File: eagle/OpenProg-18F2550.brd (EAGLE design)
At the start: 101.6 x 78.7 mm, 45 parts, among them J1 CONN-10P, J3 USB-SH, T1 BC557, T2 BC557, T3 BC547, T4 BC547, U1 PIC18F2550-I/SP-V, X1 12MHz

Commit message: ...
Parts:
- L1: value (none) -> 100µH
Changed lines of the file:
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@@
 <element name="J1" library="pinconn" package="CONN-10P" value="CONN-10P" x="78.74" y="45.72" rot="R270"/>
 <element name="J3" library="usb" package="USB-B-PRINT" value="USB-SH" x="58.42" y="11.43"/>
-<element name="L1" library="l" package="L-03/10V" value="" x="22.86" y="25.4" rot="R90"/>
+<element name="L1" library="l" package="L-03/10V" value="100µH" x="22.86" y="25.4" rot="R90"/>
 <element name="R1" library="r" package="0204/10-V" value="22kΩ" x="12.7" y="15.24" rot="R270"/>
 <element name="R10" library="r" package="0204/10" value="100kΩ" x="40.64" y="25.4"/>

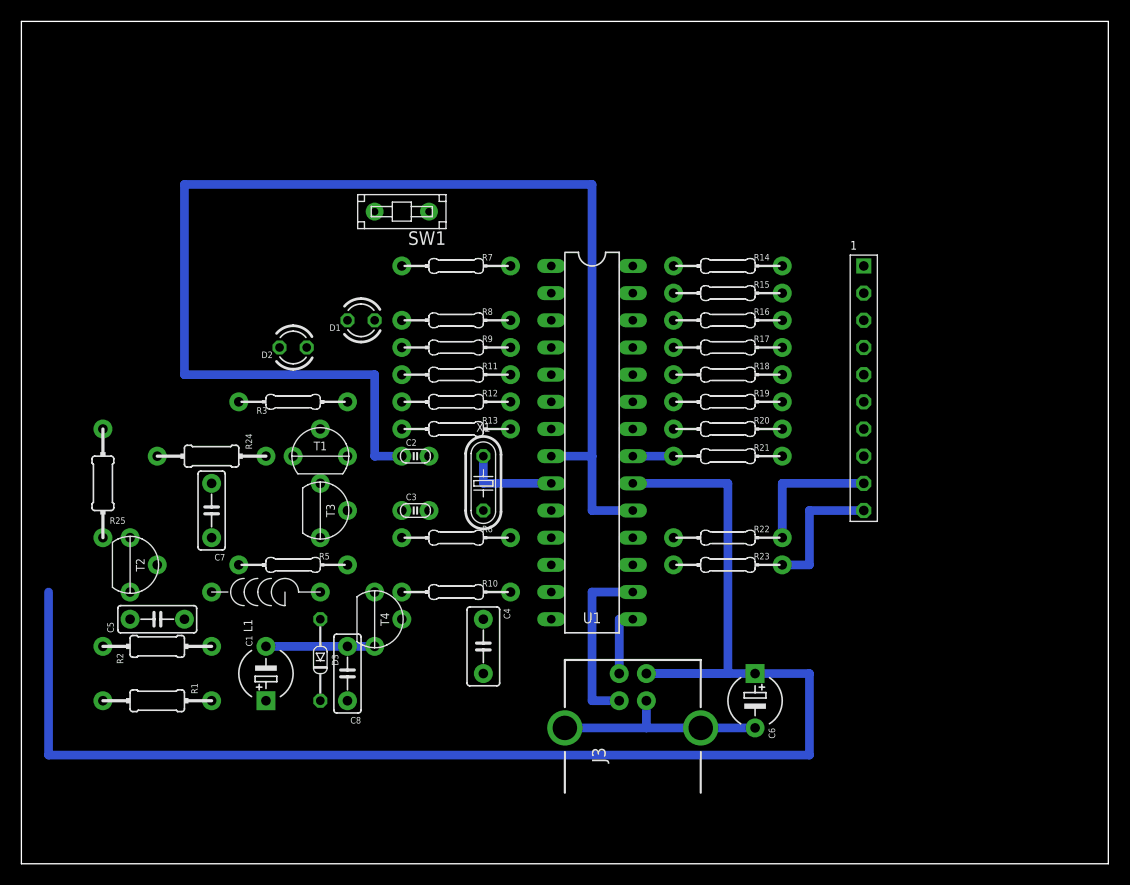
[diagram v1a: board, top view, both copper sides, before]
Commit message: ...
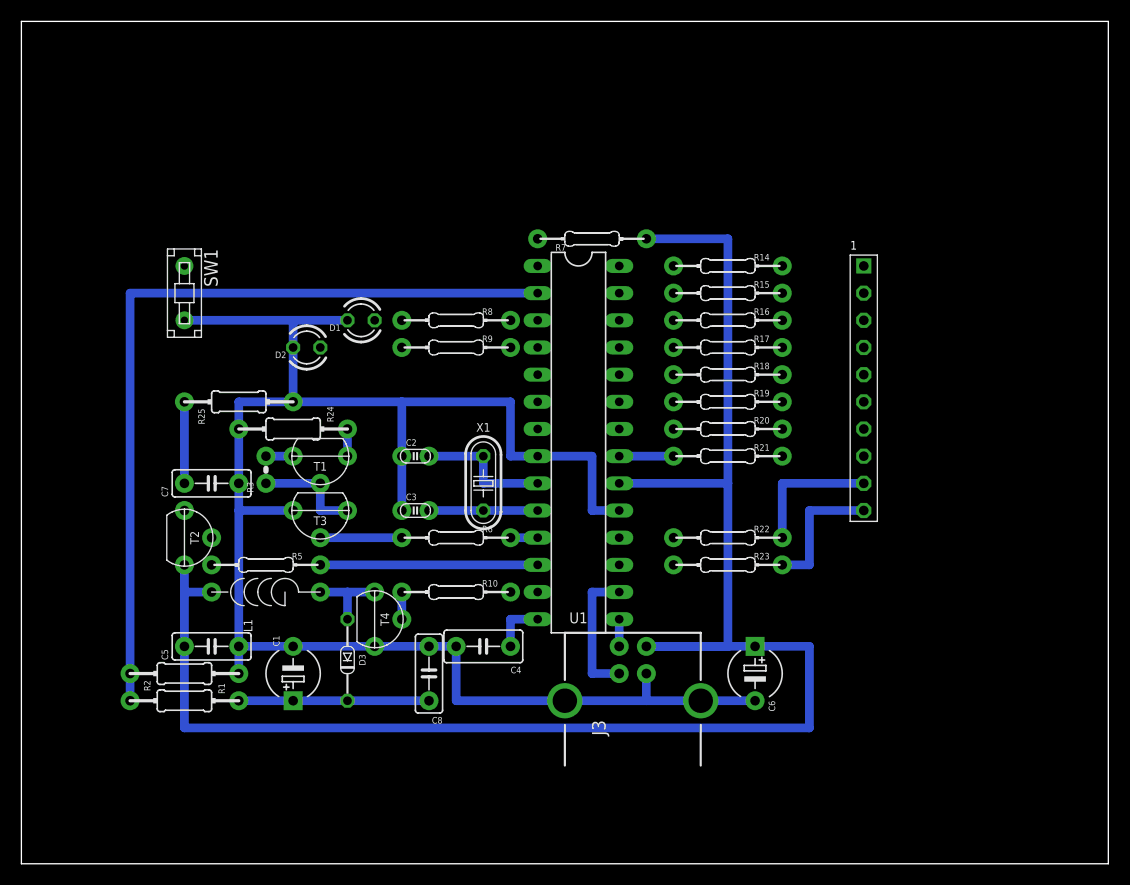
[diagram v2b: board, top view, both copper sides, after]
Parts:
- removed R11, R12, R13: 100kΩ, r:0204/10
- R3: device r:0204/10 -> r:0204/2
- moved SW1 21.7 mm to (15.2, 53.3), turned to 270 degrees
- moved R25 14.8 mm to (20.3, 43.2), turned to 90 degrees
- moved R7 13.0 mm to (53.3, 58.4), turned to 180 degrees
- moved R24 8.03 mm to (25.4, 40.6)
- moved C8 7.62 mm to (38.1, 17.8)
- moved R3 6.84 mm to (22.9, 36.8), turned to 90 degrees
- moved C5 5.68 mm to (17.8, 20.3)
- moved T2 5.68 mm to (15.2, 30.5)
- moved R2 3.59 mm to (15.2, 17.8)
- moved C6 2.54 mm to (68.6, 17.8)
- moved J3 2.54 mm to (58.4, 14.0)
- moved R1 2.54 mm to (15.2, 15.2)
- moved C1 2.54 mm to (25.4, 17.8)
- moved C7 2.54 mm to (17.8, 35.6), turned to 180 degrees
- moved D3 2.54 mm to (30.5, 19.1)
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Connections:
- removed net N$38: D1.K, D2.K, SW1.1
- removed net N$41: R7.1
- removed net RA3: R11.1
- removed net RA4: R12.1
- removed net RA5: R13.1
- net GND: now also D1.K, D2.K, SW1.1
- net N$3: no longer R11.2
- net N$4: no longer R12.2
- net N$6: no longer R13.2
- net VCC: now also R7.1
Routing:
- net FB: track 0.00 -> 76.2 mm
- net RC1: track 0.00 -> 20.3 mm
- net VCC: track 143.5 -> 162.6 mm
- net N$1: track 0.00 -> 17.8 mm
- net GND: track 153.7 -> 165.1 mm
- net N$11: track 0.00 -> 10.2 mm
- net OSC2: track 0.00 -> 10.2 mm
- net N$7: track 0.00 -> 7.62 mm
- net N$5: track 0.00 -> 7.62 mm
- net VDDU: track 0.00 -> 7.62 mm
- net N$36: track 0.00 -> 5.08 mm
- net OSC1: track 8.89 -> 12.7 mm
- net N$35: track 6.35 -> 2.54 mm
- net N$34: track 16.5 -> 12.7 mm
- net VPPU: track 0.00 -> 2.54 mm
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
